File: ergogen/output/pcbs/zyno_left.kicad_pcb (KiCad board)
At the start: 2 copper layers, 123.2 x 112 mm, 59 parts

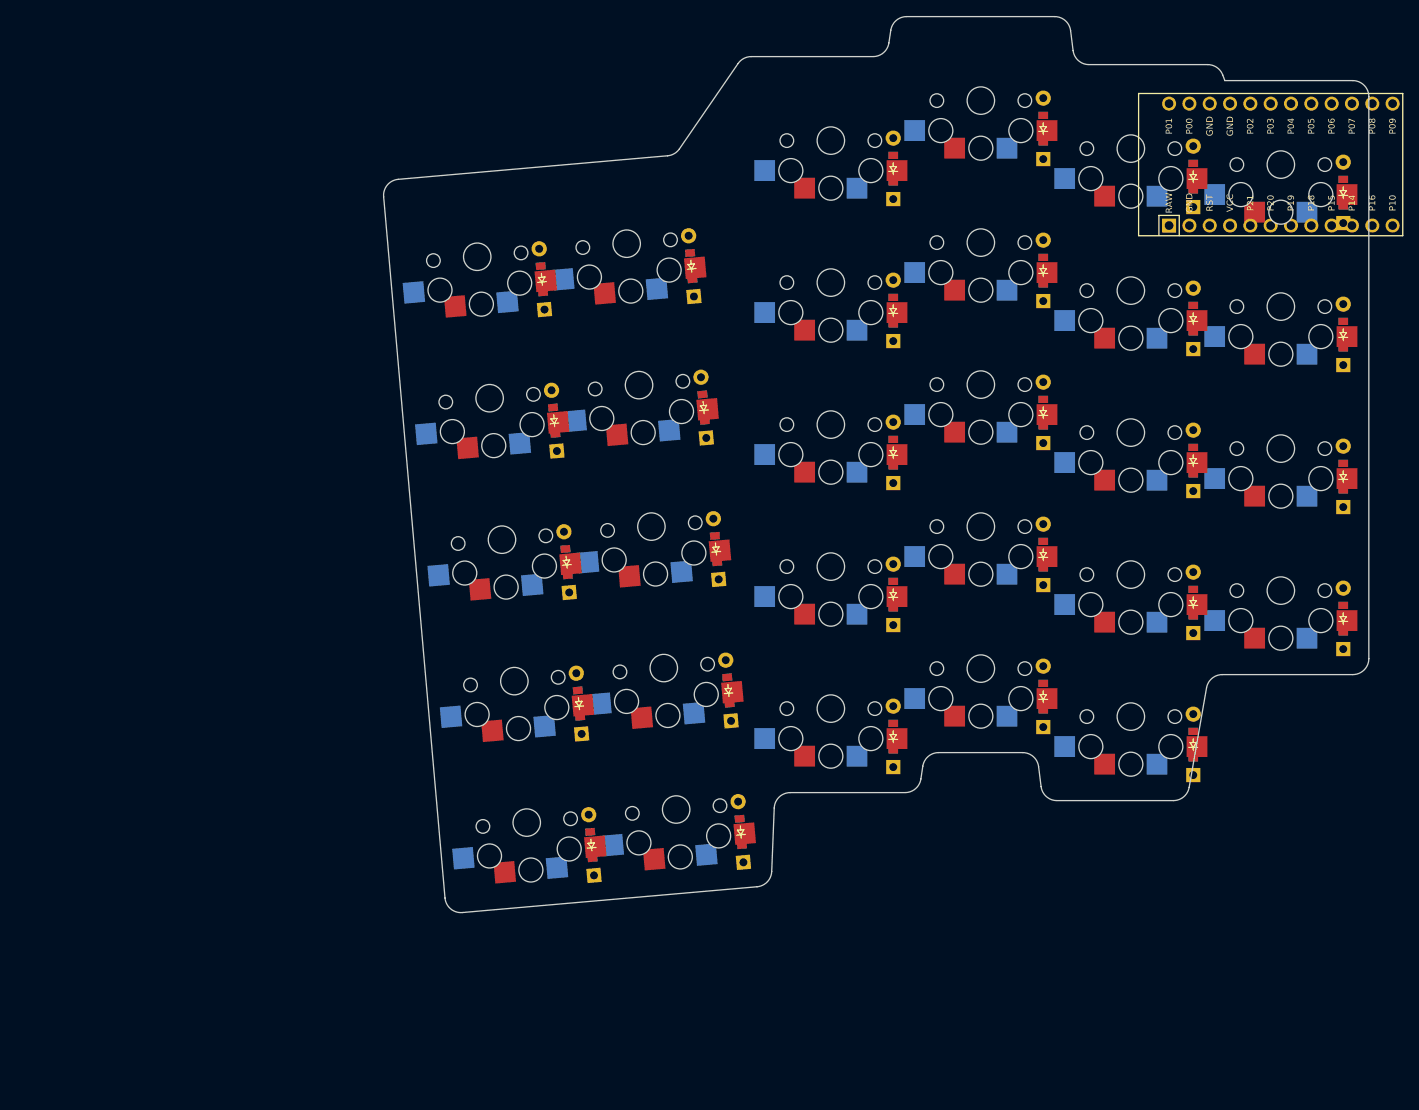
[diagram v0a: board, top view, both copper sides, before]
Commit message: ergogen done?
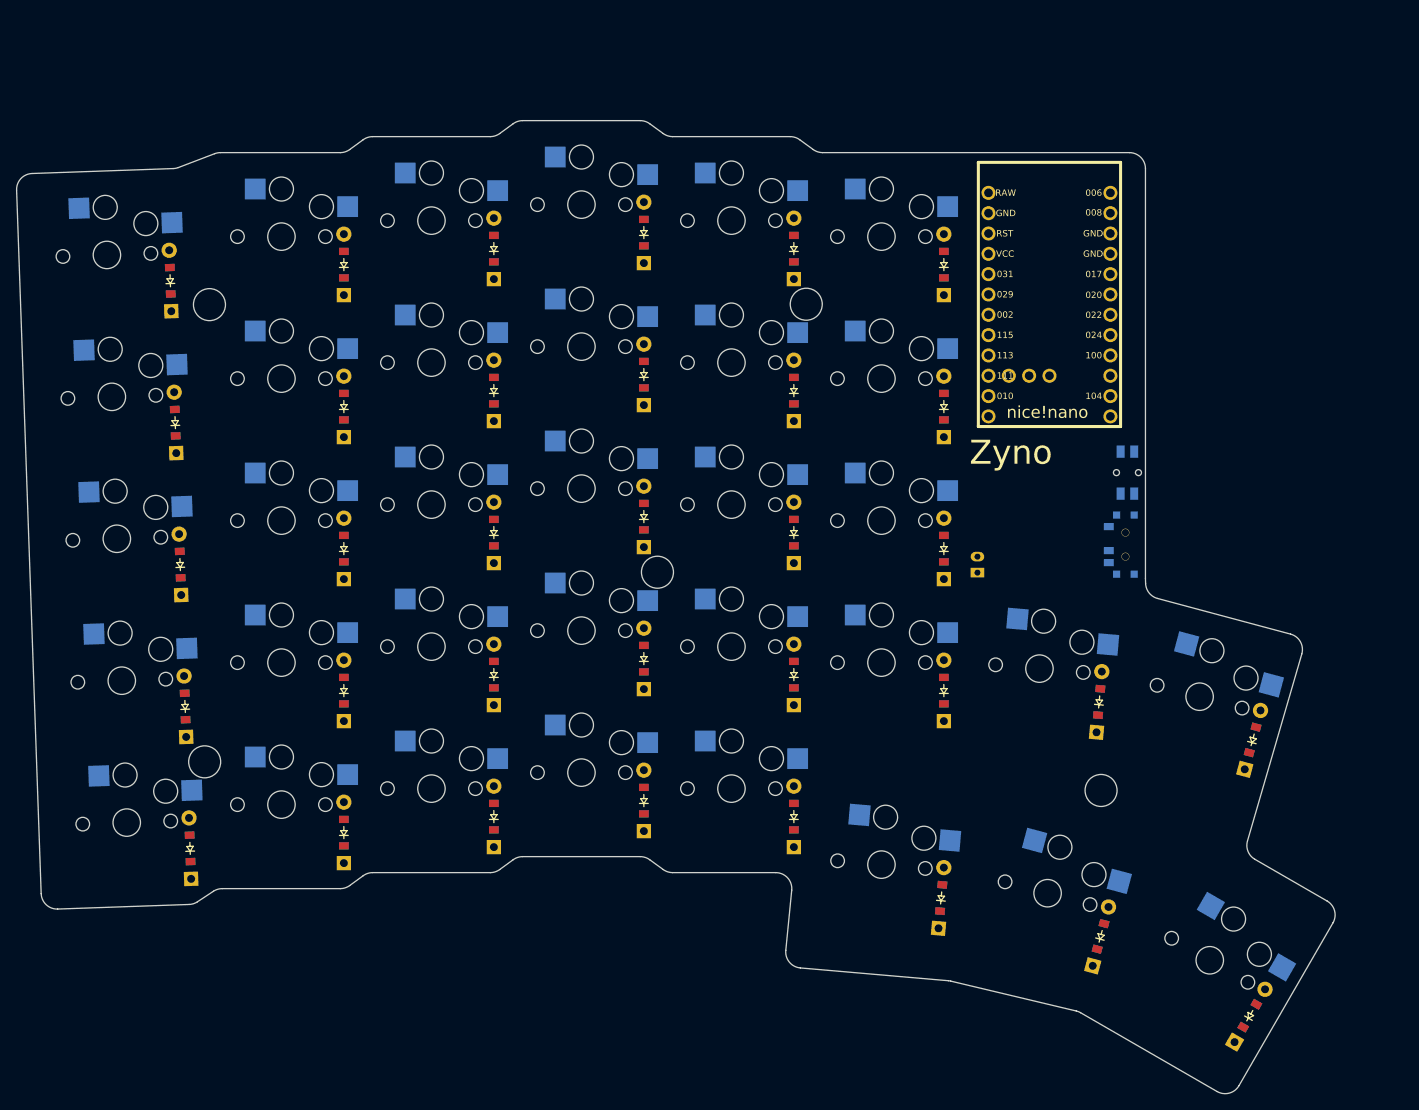
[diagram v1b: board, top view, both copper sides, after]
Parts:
- added ?: , HOLE_M2_TH, F.Cu at (171.8, 146.0)
- added ?: , HOLE_M2_TH, F.Cu at (59.7, 142.4)
- added ?: , HOLE_M2_TH, F.Cu at (60.3, 85.3)
- added ?: , HOLE_M2_TH, F.Cu at (134.9, 85.2)
- added ?: , HOLE_M2_TH, F.Cu at (116.3, 118.7)
- added B1: Panasonic_EVQPUL_EVQPUC, Panasonic_EVQPUL_EVQPUC, F.Cu at (175.1, 106.3)
- added D30: , ComboDiode, F.Cu at (151.8, 159.4)
- added D31: , ComboDiode, F.Cu at (171.7, 164.2)
- added D32: , ComboDiode, F.Cu at (190.4, 174.1)
- added D33: , ComboDiode, F.Cu at (171.6, 134.9)
- added D34: , ComboDiode, F.Cu at (190.7, 139.7)
- added JST1: , JST_PH_S2B-PH-K_02x2.00mm_Angled, F.Cu at (156.3, 117.8)
- added S30: , PG1350, F.Cu at (144.3, 155.3)
- added S31: , PG1350, F.Cu at (165.1, 158.8)
- added S32: , PG1350, F.Cu at (185.4, 167.2)
- added S33: , PG1350, F.Cu at (164.1, 130.8)
- added S34: , PG1350, F.Cu at (184.1, 134.3)
- added T1: , E73:SPDT_C128955, F.Cu at (174.8, 115.3)
- MCU1: value (none) -> nice_nano; footprint ProMicro -> nice_nano
- moved D16 51.6 mm to (114.6, 147.3)
- moved D17 51.6 mm to (114.6, 129.5)
- moved D18 51.6 mm to (114.6, 111.8)
- moved D19 51.6 mm to (114.6, 94.0)
- moved D20 51.6 mm to (114.6, 76.3)
- moved S16 51.6 mm to (106.8, 143.8), turned to 0 degrees
- moved S17 51.6 mm to (106.8, 126.0), turned to 0 degrees
- moved S18 51.6 mm to (106.8, 108.3), turned to 0 degrees
- moved S19 51.6 mm to (106.8, 90.5), turned to 0 degrees
- moved S20 51.6 mm to (106.8, 72.8), turned to 0 degrees
- moved D11 50.9 mm to (95.9, 149.3)
- moved D12 50.9 mm to (95.9, 131.5)
- moved D13 50.9 mm to (95.9, 113.8)
- moved D14 50.9 mm to (95.9, 96.0)
- moved D15 50.9 mm to (95.9, 78.3)
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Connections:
- net P0 renamed P010
- net P1 renamed P009
- D1 pad 1: (no net) -> P113
- D10 pad 1: (no net) -> P031
- D11 pad 1: (no net) -> P113
- D12 pad 1: (no net) -> P115
- D13 pad 1: (no net) -> P002
- D14 pad 1: (no net) -> P029
- D15 pad 1: (no net) -> P031
- D16 pad 1: (no net) -> P113
- D17 pad 1: (no net) -> P115
- D18 pad 1: (no net) -> P002
- D19 pad 1: (no net) -> P029
- D2 pad 1: (no net) -> P115
- D20 pad 1: (no net) -> P031
- D21 pad 1: (no net) -> P113
- D22 pad 1: (no net) -> P115
- D23 pad 1: (no net) -> P002
- D24 pad 1: (no net) -> P029
- D25 pad 1: (no net) -> P031
- D26 pad 1: (no net) -> P115
- D27 pad 1: (no net) -> P002
- D28 pad 1: (no net) -> P029
- D29 pad 1: (no net) -> P031
- D3 pad 1: (no net) -> P002
- D4 pad 1: (no net) -> P029
- D5 pad 1: (no net) -> P031
- D6 pad 1: (no net) -> P113
- D7 pad 1: (no net) -> P115
- D8 pad 1: (no net) -> P002
- D9 pad 1: (no net) -> P029
- MCU1 pad 1: RAW -> P006
- MCU1 pad 10: P14 -> P011
- MCU1 pad 11: P16 -> P104
- MCU1 pad 12: P10 -> P106
- MCU1 pad 15: GND -> P111
- MCU1 pad 16: GND -> P113
- MCU1 pad 17: P2 -> P115
- MCU1 pad 18: P3 -> P002
- MCU1 pad 19: P4 -> P029
- MCU1 pad 2: GND -> P008
- MCU1 pad 20: P5 -> P031
- MCU1 pad 21: P6 -> VCC
- MCU1 pad 22: P7 -> RST
- MCU1 pad 23: P8 -> GND
- MCU1 pad 24: P9 -> RAW
- MCU1 pad 3: RST -> GND
- MCU1 pad 4: VCC -> GND
- MCU1 pad 5: P21 -> P017
- MCU1 pad 6: P20 -> P020
- MCU1 pad 7: P19 -> P022
- MCU1 pad 8: P18 -> P024
- MCU1 pad 9: P15 -> P100
- S1 pad 1: (no net) -> P020
- S10 pad 1: (no net) -> P022
- S11 pad 1: (no net) -> P024
- S12 pad 1: (no net) -> P024
- S13 pad 1: (no net) -> P024
- S14 pad 1: (no net) -> P024
- S15 pad 1: (no net) -> P024
- S16 pad 1: (no net) -> P100
- S17 pad 1: (no net) -> P100
- S18 pad 1: (no net) -> P100
- S19 pad 1: (no net) -> P100
- S2 pad 1: (no net) -> P020
- S20 pad 1: (no net) -> P100
- S21 pad 1: (no net) -> P011
- S22 pad 1: (no net) -> P011
- S23 pad 1: (no net) -> P011
- S24 pad 1: (no net) -> P011
- S25 pad 1: (no net) -> P011
- S26 pad 1: (no net) -> P017
- S27 pad 1: (no net) -> P017
- S28 pad 1: (no net) -> P017
- S29 pad 1: (no net) -> P017
- S3 pad 1: (no net) -> P020
- S4 pad 1: (no net) -> P020
- S5 pad 1: (no net) -> P020
- S6 pad 1: (no net) -> P022
- S7 pad 1: (no net) -> P022
- S8 pad 1: (no net) -> P022
- S9 pad 1: (no net) -> P022
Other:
- board size 123.2 x 112 mm -> 164.8 x 121.6 mm
- board text added: "Zyno"
